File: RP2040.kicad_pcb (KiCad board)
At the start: 2 copper layers, 21 x 51 mm, 41 parts, among them J1 USB_C_Receptacle_USB2.0_14P, J2 Conn_01x20, J3 Conn_01x20, J4 Conn_01x03, SW1 SW_Push, U1 RP2040, U2 MCP1700x-330xxTT, U4 W25Q16JVUXIQ TR, Y1 12 MHz

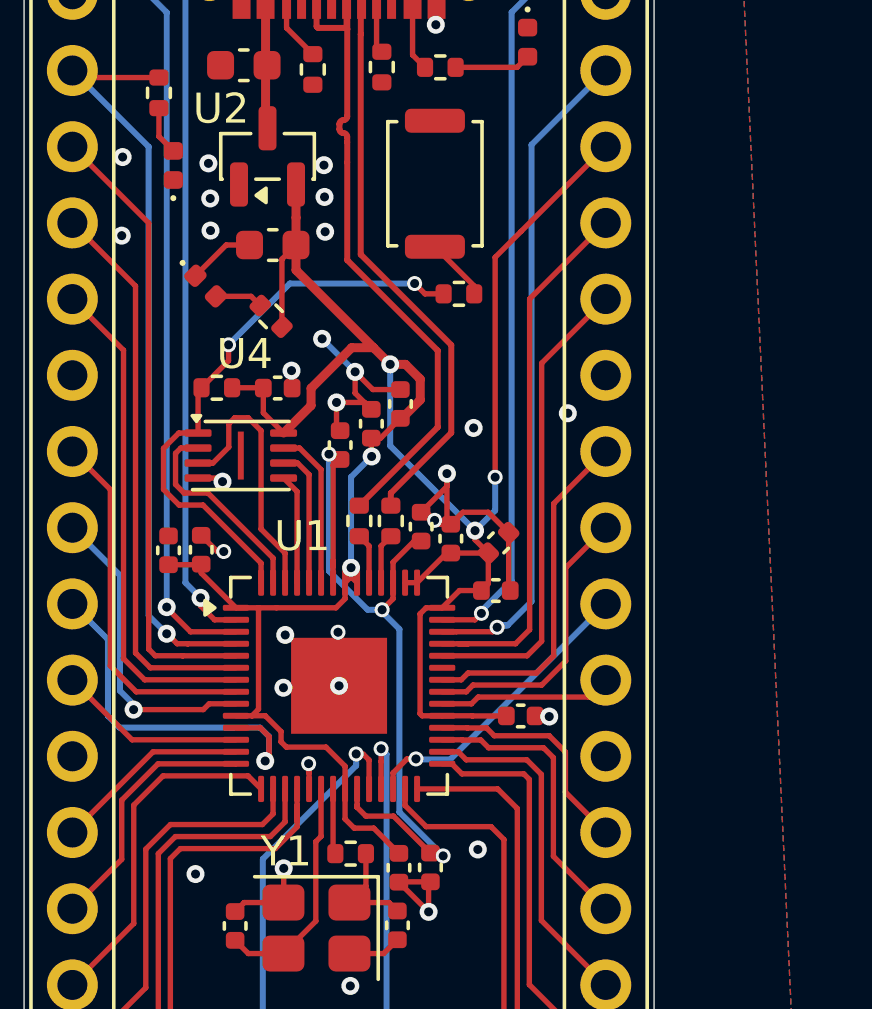
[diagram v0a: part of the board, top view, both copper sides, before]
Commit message: Update Readme
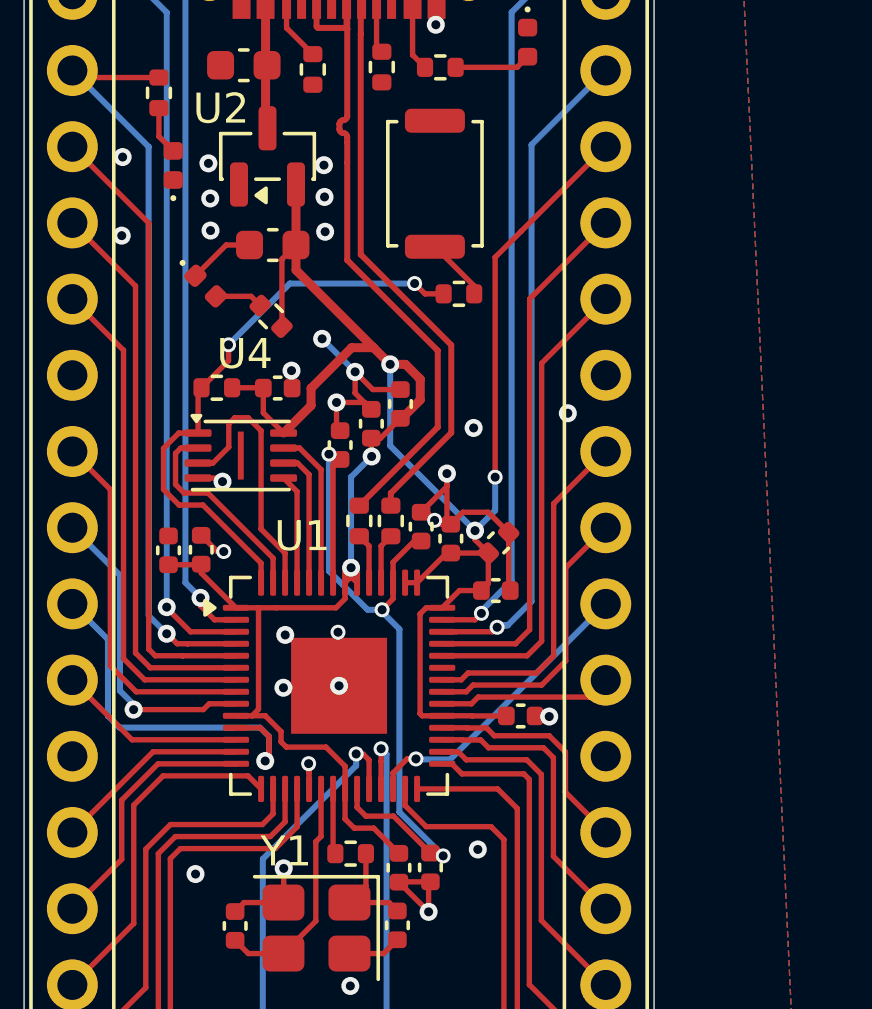
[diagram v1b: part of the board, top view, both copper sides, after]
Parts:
- R10: value 1k -> 470
- R8, R9: value 330 -> 100
- moved G*** 0.36 mm to (172.7, 56.2)
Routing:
- net GPIO15: track 22.2 -> 21.7 mm
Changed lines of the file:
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@@
 			)
 		)
-		(property "Value" "1k"
+		(property "Value" "470"
 			(at 0 1.17 0)
 			(layer "F.Fab")
@@
 			)
 		)
-		(property "Value" "330"
+		(property "Value" "100"
 			(at 0 1.17 135)
 			(layer "F.Fab")
@@
 		)
 		(embedded_fonts no)
-		(model "${KICAD9_3DMODEL_DIR}/Connector_USB.3dshapes/USB_C_Receptacle_HRO_TYPE-C-31-M-12.step"
+		(model "${KICAD9_3DMODEL_DIR}/Connector_USB.3dshapes/User Library-664121_1623983041_9594.step"
+			(hide yes)
+			(offset
+				(xyz -4.2 3.6 3)
+			)
+			(scale
+				(xyz 1 1 1)
+			)
+			(rotate
+				(xyz -180 -90 -0)
+			)
+		)
+		(model "${KICAD9_3DMODEL_DIR}/Connector_USB.3dshapes/USB_C_Receptacle_GCT_USB4105-xx-A_16P_TopMnt_Horizontal.wrl"
 			(offset
 				(xyz 0 0 0)
@@
 			)
 		)
-		(property "Value" "330"
+		(property "Value" "100"
 			(at 0 1.17 90)
 			(layer "F.Fab")
@@
 	(footprint "assets:stem_logo_large"
 		(layer "B.Cu")
-		(at 173 56.1 180)
+		(at 172.67 56.25 180)
 		(property "Reference" "G***"
 			(at 0 0 0)
@@
 	)
 	(segment
-		(start 171.34 58.465)
-		(end 171.34 59.57)
-		(width 0.3)
-		(layer "F.Cu")
-		(net 2)
-	)
-	(segment
 		(start 173.85 66.92)
 		(end 173.85 67.52)
@@
 	)
 	(segment
-		(start 171.291 59.521)
-		(end 171.34 59.57)
-		(width 0.18)
-		(layer "F.Cu")
-		(net 2)
-	)
-	(segment
 		(start 178.84 60.03)
 		(end 177.977 60.893)
@@
 	)
 	(segment
+		(start 171.34 58.465)
+		(end 171.34 60.4825)
+		(width 0.3)
+		(layer "F.Cu")
+		(net 2)
+	)
+	(segment
 		(start 176.5 70.75)
 		(end 176.3625 70.75)
@@
 	)
 	(segment
-		(start 171.34 59.57)
-		(end 171.34 60.4825)
-		(width 0.3)
-		(layer "F.Cu")
-		(net 2)
-	)
-	(segment
 		(start 174.98826 64.46)
 		(end 174.48 64.46)
@@
 	)
 	(segment
-		(start 173.376 79.226)
-		(end 173.376 79.148774)
+		(start 173.375 79.225)
+		(end 173.669 79.519)
 		(width 0.18)
 		(layer "F.Cu")
@@
 	)
 	(segment
-		(start 172.575 71.011)
-		(end 172.576 71.01)
-		(width 0.18)
-		(layer "F.Cu")
-		(net 3)
-	)
-	(segment
-		(start 172.576 67.824)
-		(end 172.576 71.01)
-		(width 0.18)
-		(layer "F.Cu")
-		(net 3)
-	)
-	(segment
 		(start 172.437983 67.452266)
 		(end 172.632266 67.452266)
@@
 	)
 	(segment
-		(start 173.375 79.225)
-		(end 173.376 79.226)
-		(width 0.18)
-		(layer "F.Cu")
-		(net 3)
-	)
-	(segment
-		(start 172.575 71.7375)
-		(end 172.575 71.011)
+		(start 172.575 67.865)
+		(end 172.81 67.63)
 		(width 0.18)
 		(layer "F.Cu")
@@
 	)
 	(segment
-		(start 173.669 79.519)
-		(end 173.376 79.226)
-		(width 0.18)
-		(layer "F.Cu")
-		(net 3)
-	)
-	(segment
 		(start 173.375 78.6125)
 		(end 173.375 79.225)
@@
 	)
 	(segment
-		(start 172.576 71.01)
-		(end 172.576 71.201226)
+		(start 172.81 67.63)
+		(end 172.77 67.63)
 		(width 0.18)
 		(layer "F.Cu")
@@
 	)
 	(segment
-		(start 172.81 67.63)
-		(end 172.77 67.63)
+		(start 172.575 71.7375)
+		(end 172.575 67.865)
 		(width 0.18)
 		(layer "F.Cu")
@@
 	)
 	(segment
-		(start 171.375 78.6125)
-		(end 171.375 79.678)
+		(start 171.375 79.87275)
+		(end 171.377 79.87475)
 		(width 0.18)
 		(layer "F.Cu")
@@
 	)
 	(segment
-		(start 171.377 79.68)
-		(end 171.377 79.149774)
-		(width 0.18)
-		(layer "F.Cu")
-		(net 11)
-	)
-	(segment
-		(start 171.377 79.87475)
-		(end 171.377 79.68)
-		(width 0.18)
-		(layer "F.Cu")
-		(net 11)
-	)
-	(segment
 		(start 167.151 80.9361)
 		(end 167.4851 80.602)
@@
 	)
 	(segment
-		(start 171.375 79.678)
-		(end 171.377 79.68)
+		(start 171.375 78.6125)
+		(end 171.375 79.87275)
 		(width 0.18)
 		(layer "F.Cu")
@@
 	)
 	(segment
-		(start 177.07 73.774)
-		(end 176.748774 73.774)
-		(width 0.18)
-		(layer "F.Cu")
-		(net 40)
-	)
-	(segment
-		(start 179.127 73.303)
-		(end 178.656 73.774)
+		(start 178.655 73.775)
+		(end 179.127 73.303)
 		(width 0.18)
 		(layer "F.Cu")
@@
 	(segment
 		(start 176.2125 73.775)
-		(end 177.069 73.775)
+		(end 178.655 73.775)
 		(width 0.18)
 		(layer "F.Cu")
@@
 	)
 	(segment
-		(start 178.656 73.774)
-		(end 177.07 73.774)
+		(start 179.127 62.283)
+		(end 181.665 59.745)
 		(width 0.18)
 		(layer "F.Cu")
@@
 	)
 	(segment
-		(start 181.665 59.745)
+		(start 179.127 73.303)
 		(end 179.127 62.283)
 		(width 0.18)
@@
 	)
 	(segment
-		(start 177.069 73.775)
-		(end 177.07 73.774)
-		(width 0.18)
-		(layer "F.Cu")
-		(net 40)
-	)
-	(segment
-		(start 179.127 62.283)
-		(end 179.127 73.303)
-		(width 0.18)
-		(layer "F.Cu")
-		(net 40)
-	)
-	(segment
 		(start 173.571663 77.446669)
 		(end 173.775 77.650006)
@@
 			(thermal_gap 0.3)
 			(thermal_bridge_width 0.5)
-			(island_removal_mode 1)
-			(island_area_min 10)
 		)
 		(polygon

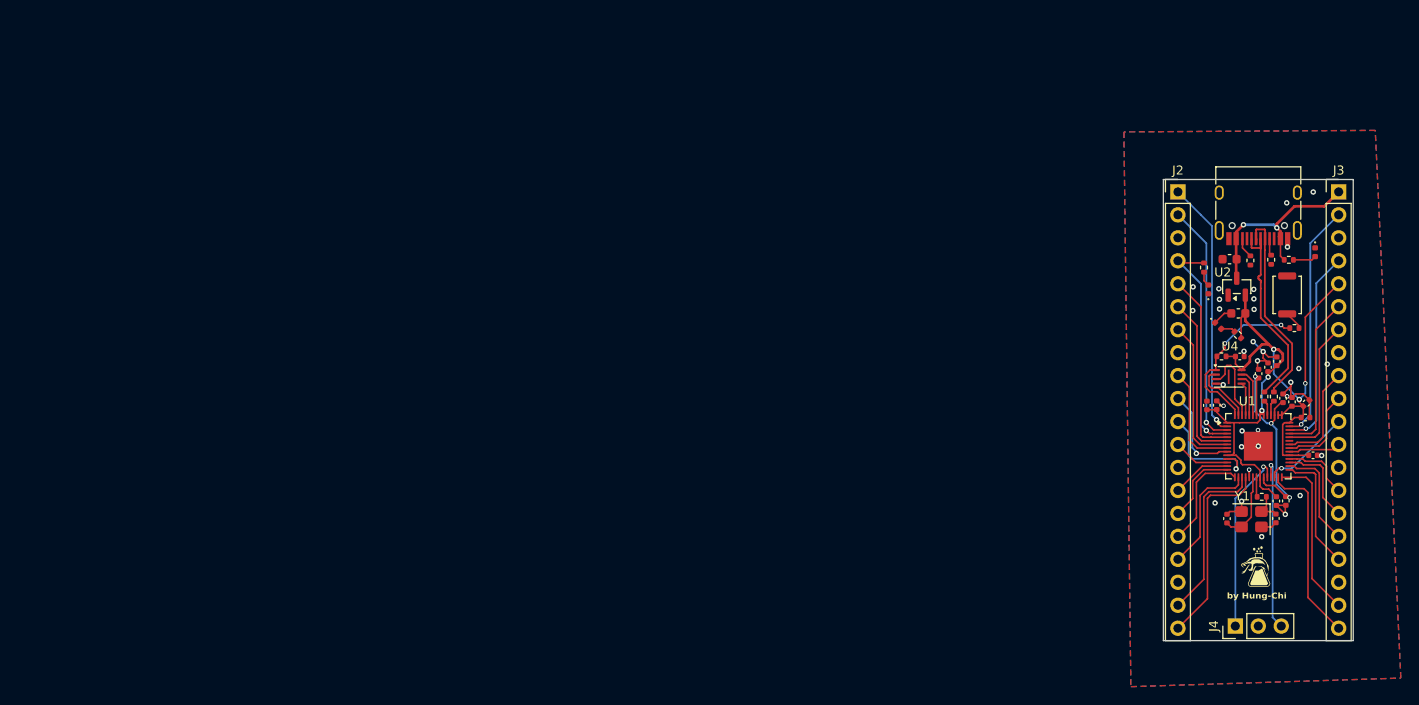
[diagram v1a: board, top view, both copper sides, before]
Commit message: Update Readme + Images
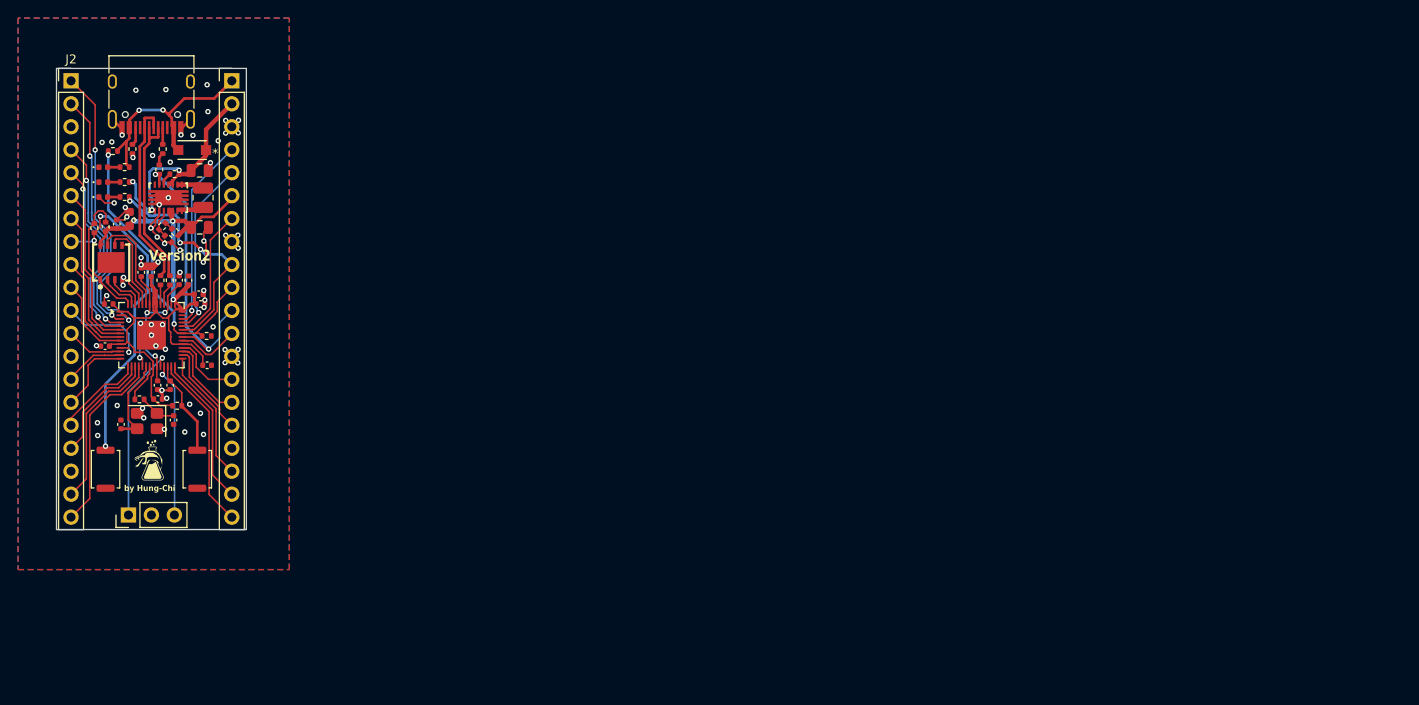
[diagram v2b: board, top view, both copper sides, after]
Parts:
- removed C16: 33pF, Capacitor_SMD:C_0402_1005Metric
- removed the G*** at (172.7, 56.2)
- removed U4: W25Q16JVUXIQ TR, Package_SON:Winbond_USON-8-1EP_3x2mm_P0.5mm_EP0.2x1.6mm
- added 111111111: MBR120VLSFT1G, RP2040:SDO_SOD-123FL_ONS, F.Cu at (54.9, 42.4)
- added C18: 0.1uF, Capacitor_SMD:C_0402_1005Metric, F.Cu at (45.2, 64.1)
- added C19: 0.1uF, Capacitor_SMD:C_0402_1005Metric, F.Cu at (50.3, 55.9)
- added L1: 2u2, Inductor_SMD:L_1008_2520Metric, F.Cu at (56.1, 47.7)
- added R11: 100K, Resistor_SMD:R_0402_1005Metric, F.Cu at (51.2, 44.6)
- added R12: 10K, Resistor_SMD:R_0402_1005Metric, F.Cu at (53.2, 70.7)
- added R13: 1K, Resistor_SMD:R_0402_1005Metric, F.Cu at (49.0, 70.0)
- added R14: 27, Resistor_SMD:R_0402_1005Metric, F.Cu at (51.4, 56.8)
- added R15: 27, Resistor_SMD:R_0402_1005Metric, F.Cu at (52.4, 56.8)
- added R16: 330, Resistor_SMD:R_0402_1005Metric, F.Cu at (47.4, 46.0)
- added R17: 330, Resistor_SMD:R_0402_1005Metric, F.Cu at (47.4, 47.6)
- added R18: 1K, Resistor_SMD:R_0402_1005Metric, F.Cu at (47.4, 44.3)
- added SW2: SW_Push, Button_Switch_SMD:SW_Push_SPST_NO_Alps_SKRK, F.Cu at (55.4, 77.7)
- added U1: RT6154AGQW, easyeda2kicad:VSON-14_L4.0-W3.0-P0.50-BL-EP_TI_DSJ, F.Cu at (52.2, 47.7)
- C1, C10: value 1uF -> 0.1uF
- C11, C8: value 0.1uF -> 1uF
- C13, C14: value 10uF -> 0.1uF; footprint Capacitor_SMD:C_0603_1608Metric -> Capacitor_SMD:C_0402_1005Metric
- C15: value 33pF -> 0.1uF
- C2: value 0.1uF -> 2u2; footprint Capacitor_SMD:C_0402_1005Metric -> Capacitor_SMD:C_0603_1608Metric
- C3, C4: value 0.1uF -> 47uF; footprint Capacitor_SMD:C_0402_1005Metric -> Capacitor_SMD:C_0805_2012Metric
- C5, C6: value 0.1uF -> 15pF
- R1: value 5.1K -> 10K
- R10: value 470 -> 180K
- R3: value 27 -> 330K
- R4: value 27 -> 1K
- R5: value 1K -> 5K6
- R6: value 1K -> 100K
- R7: value 10K -> 5.1K
- R8: value 100 -> 680K
- R9: value 100 -> 10K
- U2: value MCP1700x-330xxTT -> W25Q64JVXGIQ; footprint Package_TO_SOT_SMD:SOT-23 -> easyeda2kicad:XSON-8_L4.0-W4.0-P0.80-TL-EP
- moved D3 134.4 mm to (45.0, 44.3), turned to 0 degrees
- moved C1 133.1 mm to (46.5, 50.6), turned to 90 degrees
- moved R5 132.7 mm to (46.1, 42.5)
- moved SW1 132.1 mm to (45.3, 77.7), turned to 90 degrees
- moved C2 131.9 mm to (47.9, 50.0), turned to 90 degrees
- moved R4 131.8 mm to (44.0, 51.1), turned to 90 degrees
- moved C12 130.3 mm to (45.6, 59.4), turned to 180 degrees
- moved R1 129.0 mm to (45.3, 50.9), turned to 90 degrees
- moved C7 126.6 mm to (52.4, 68.4), turned to 90 degrees
- moved C9 126.0 mm to (49.2, 55.9)
- moved R6 125.0 mm to (52.9, 45.1)
- moved U2 124.5 mm to (45.9, 54.9)
- moved D2 124.1 mm to (45.0, 47.6), turned to 0 degrees
- moved R10 124.0 mm to (52.2, 52.3), turned to -45 degrees
- moved C11 123.8 mm to (54.4, 56.8), turned to 90 degrees
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- renumbered U1 to U3
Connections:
- C11 pad 1: +1V1 -> +3V3
- C12 pad 1: +1V1 -> +3V3
- C13 pad 1: VBUS -> +3V3
- C15 pad 1: GND -> +3V3
- C15 pad 2: XIN -> GND
- C4 pad 1: +3V3 -> VSYS
- C5 pad 1: +3V3 -> GND
- C5 pad 2: GND -> XIN
- C6 pad 1: +3V3 -> GND
- C6 pad 2: GND -> Net-(C6-Pad2)
- C7 pad 1: +3V3 -> GND
- C7 pad 2: GND -> Net-(U3-RUN)
- C8 pad 1: +3V3 -> +1V1
- C9 pad 1: +3V3 -> +1V1
- J2 pad 8: GND -> BOOTSEL
- J3 pad 10: GPIO23 -> GPIO24
- J3 pad 11: RUN -> GPIO23
- J3 pad 17: GPIO18 -> GND
- J3 pad 18: GND -> GPIO18
- J3 pad 2: GPIO29_ADC3 -> VSYS
- J3 pad 5: +3V3 -> GPIO27_ADC1
- J3 pad 6: GPIO27_ADC1 -> +3V3
- J3 pad 9: GPIO24 -> GPIO25
- R1 pad 1: Net-(J1-CC1) -> +3V3
- R1 pad 2: GND -> QSPI_SS
- R10 pad 1: VBUS -> Net-(U1-FB)
- R10 pad 2: Net-(D3-A) -> GND
- R2 pad 1: Net-(J1-CC2) -> Net-(J1-CC1)
- R3 pad 1: USB_D+ -> +3V3
- R3 pad 2: Net-(U1-USB_DP) -> Net-(R3-Pad2)
- R4 pad 1: USB_D- -> BOOTSEL
- R4 pad 2: Net-(U1-USB_DM) -> QSPI_SS
- R5 pad 1: Net-(C16-Pad2) -> VBUS
- R5 pad 2: XOUT -> GPIO24
- R6 pad 1: Net-(R6-Pad1) -> VSYS
- R6 pad 2: QSPI_SS -> Net-(U1-EN)
- R7 pad 1: +3V3 -> Net-(J1-CC2)
- R7 pad 2: QSPI_SS -> GND
- R8 pad 1: GPIO2 -> Net-(R3-Pad2)
- R8 pad 2: Net-(D1-A) -> Net-(U1-FB)
- R9 pad 1: +3V3 -> GPIO24
- R9 pad 2: Net-(D2-A) -> GND
- SW1 pad 2: Net-(R6-Pad1) -> BOOTSEL
- U2 pad 1: GND -> QSPI_SS
- U2 pad 2: +3V3 -> QSPI_SD1
- U2 pad 3: VBUS -> QSPI_SD2
- U3 pad 26: RUN -> Net-(U3-RUN)
- U3 pad 37: unconnected-(U1-GPIO25-Pad37) -> GPIO25
- U3 pad 41: GPIO29_ADC3 -> unconnected-(U3-GPIO29_ADC3-Pad41)
- U3 pad 46: Net-(U1-USB_DM) -> Net-(U3-USB_DM)
- U3 pad 47: Net-(U1-USB_DP) -> Net-(U3-USB_DP)
- Y1 pad 1: Net-(C16-Pad2) -> Net-(C6-Pad2)
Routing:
- net BOOTSEL: track 0.00 -> 36.0 mm, vias 0 -> 3
- net GND: track 31.3 -> 62.2 mm, vias 32 -> 68
- net GPIO25: track 0.00 -> 28.1 mm, vias 0 -> 3
- net GPIO29_ADC3: track 26.3 -> 0.00 mm, vias 1 -> 0
- net GPIO23: track 9.54 -> 32.2 mm, vias 0 -> 2
- net VSYS: track 0.00 -> 22.0 mm, vias 0 -> 2
- net GPIO24: track 11.6 -> 32.9 mm, vias 0 -> 2
- net Net-(U3-RUN): track 0.00 -> 10.6 mm
- net RUN: track 9.97 -> 0.00 mm, vias 1 -> 0
- net +1V1: track 27.3 -> 18.5 mm
- net +3V3: track 82.1 -> 88.8 mm, vias 5 -> 4
- net QSPI_SD3: track 5.32 -> 11.4 mm
- net QSPI_SCLK: track 4.61 -> 9.84 mm
- net QSPI_SD2: track 8.76 -> 4.26 mm
- net QSPI_SS: track 19.2 -> 15.0 mm, vias 2 -> 0
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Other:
- board text added: "*"
- board text added: "3V3"
- board text added: "GND"
- board text added: "GP0"
- board text added: "GP1"
- board text added: "GP10"
- board text added: "GP11"
- board text added: "GP12"
- board text added: "GP13"
- board text added: "GP14"
- board text added: "GP15"
- board text added: "GP16"
- board text added: "GP17"
- board text added: "GP18"
- board text added: "GP19"
- board text added: "GP2"
- board text added: "GP20"
- board text added: "GP21"
- board text added: "GP22"
- board text added: "GP23"
- board text added: "GP24"
- board text added: "GP26_A0"
- board text added: "GP27_A1"
- board text added: "GP28_A2"
- board text added: "GP3"
- board text added: "GP4"
- board text added: "GP5"
- board text added: "GP6"
- board text added: "GP7"
- board text added: "GP8"
- board text added: "GP9"
- board text added: "RUN"
- board text added: "VBUS"
- board text added: "VYSY"
- board text added: "Version2"

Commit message: update image
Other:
- board text added: "BOOTSEL"
- board text added: "GP25"
- board text added: "GP26_ADC0"
- board text added: "GP27_ADC1"
- board text added: "GP28_ADC2"
- board text added: "SWCLK"
- board text added: "SWD"
- board text added: "VSYS"
- board text removed: "By Hung-Chi"
- board text removed: "GP26_A0"
- board text removed: "GP27_A1"
- board text removed: "GP28_A2"
- board text removed: "RUN"
- board text removed: "VYSY"
